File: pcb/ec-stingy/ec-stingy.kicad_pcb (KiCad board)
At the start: 2 copper layers, 52 parts, among them J1 PJ-320D-A, J2 Conn_01x02_Male, J3 Conn_01x04_Male, J4 105133-0011, SW1 PCM12SMTR, U1 AD8232, U2 STM32F334R8T6, U3 CP2102N-A02-GQFN20R, Y1 16MHz

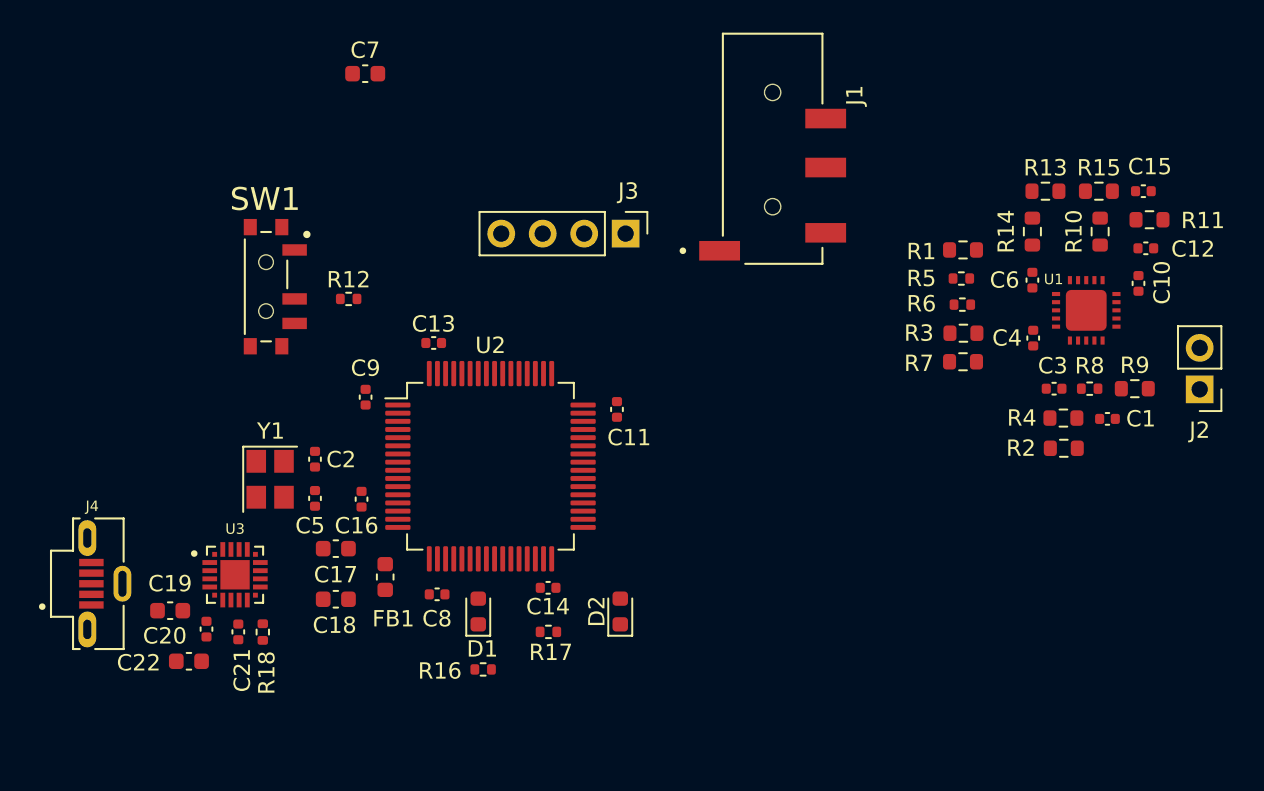
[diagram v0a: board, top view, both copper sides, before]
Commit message: more pcb progress
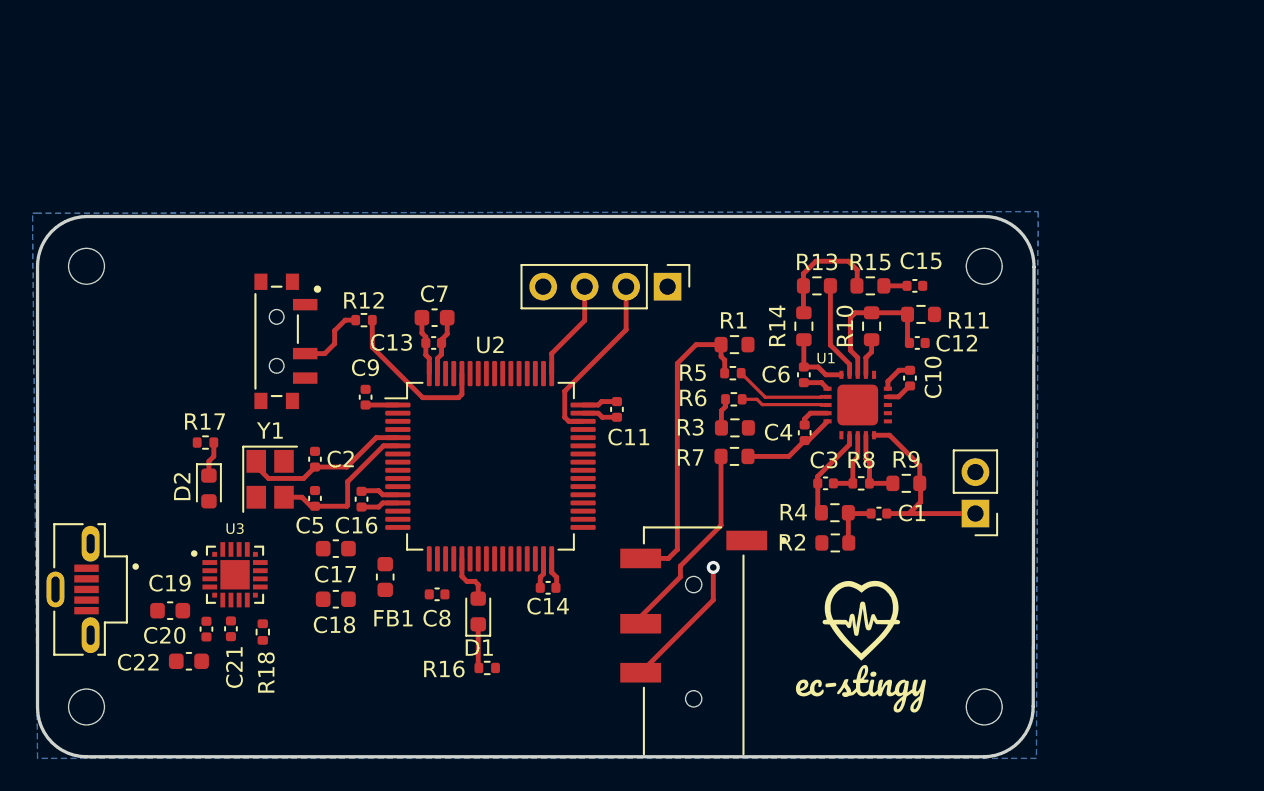
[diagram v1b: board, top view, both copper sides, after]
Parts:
- added G***: LOGO, LOGO, F.Cu at (65.0, 50.7)
- added H1: MountingHole, MountingHole:MountingHole_2.2mm_M2, F.Cu at (17.5, 54.4)
- added H2: MountingHole, MountingHole:MountingHole_2.2mm_M2, F.Cu at (72.5, 54.4)
- added H3: MountingHole, MountingHole:MountingHole_2.2mm_M2, F.Cu at (72.5, 27.4)
- added H4: MountingHole, MountingHole:MountingHole_2.2mm_M2, F.Cu at (17.5, 27.4)
- moved J1 30.5 mm to (54.7, 50.4), turned to 90 degrees
- moved D2 26.3 mm to (25.0, 41.0), turned to -90 degrees
- moved R17 24.0 mm to (24.8, 38.1)
- moved J2 15.7 mm to (72.0, 42.5)
- moved C7 15.5 mm to (38.8, 30.5)
- moved C1 15.2 mm to (66.0, 42.5)
- moved C10 15.2 mm to (68.0, 34.2)
- moved C12 15.2 mm to (68.4, 32.0)
- moved C15 15.2 mm to (68.2, 28.6)
- moved C3 15.2 mm to (62.8, 40.6)
- moved C4 15.2 mm to (61.5, 37.5)
- moved C6 15.2 mm to (61.5, 34.0)
- moved R1 15.2 mm to (57.2, 32.1)
- moved R10 15.2 mm to (65.6, 31.0)
- moved R11 15.2 mm to (68.6, 30.3)
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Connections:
- net /+IN renamed /IN+
- net /-IN renamed /IN-
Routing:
- net /LA: track 0.00 -> 18.9 mm
- net +3.3V: track 0.00 -> 14.0 mm
- net /ADC1_IN1: track 0.00 -> 12.6 mm
- net /RL: track 0.00 -> 12.3 mm
- net GND: track 0.00 -> 11.7 mm
- net /TMS: track 0.00 -> 10.8 mm
- net /RCC_OSC_IN: track 0.00 -> 10.3 mm
- net /RA: track 0.00 -> 10.1 mm, vias 0 -> 1
- net /BOOT0: track 0.00 -> 9.79 mm
- net /RCC_OSC_OUT: track 0.00 -> 9.59 mm
- net /REFIN: track 0.00 -> 9.15 mm
- net Net-(R13-Pad1): track 0.00 -> 7.22 mm
- net /TCK: track 0.00 -> 6.16 mm
- net /IAOUT: track 0.00 -> 5.94 mm
- net /IN+: track 0.00 -> 5.91 mm
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- added copper zone on B.Cu, net GND
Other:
- board outline added: 61 x 33.1 mm
